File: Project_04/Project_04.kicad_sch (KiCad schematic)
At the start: 1 part, among them U1 74AUC2G79

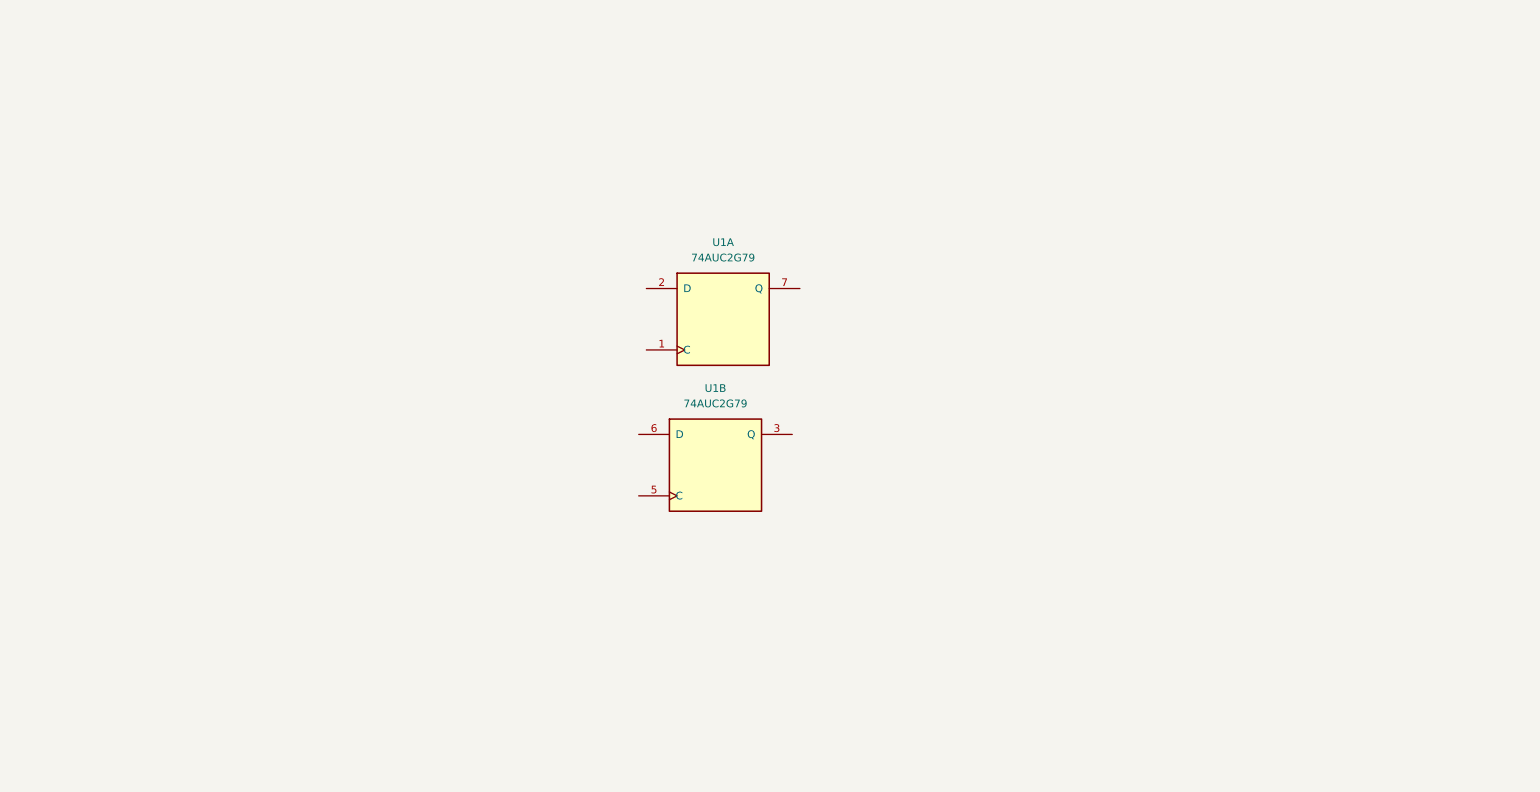
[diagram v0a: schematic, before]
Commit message: some changes
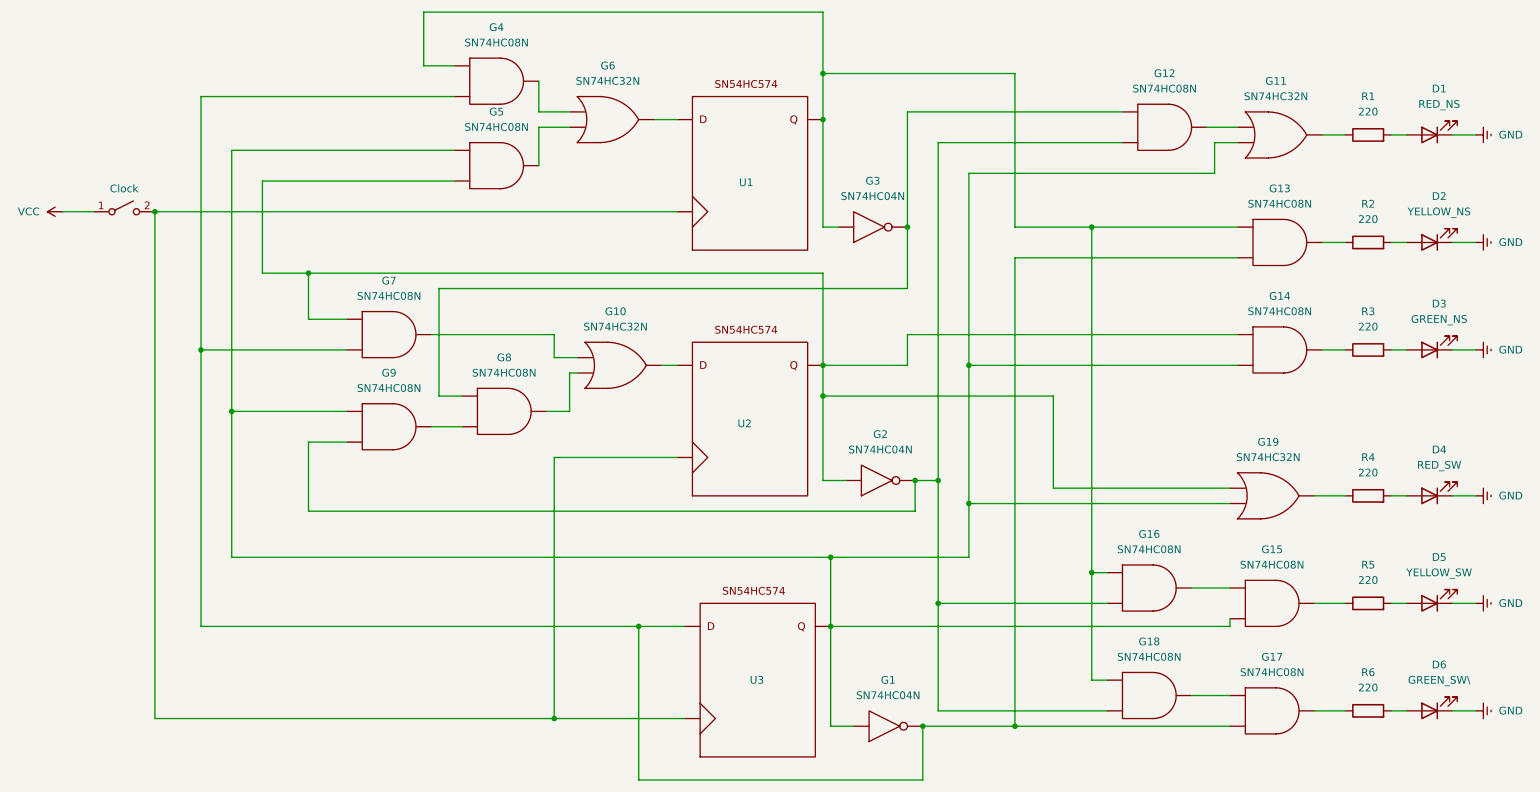
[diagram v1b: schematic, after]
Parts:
- removed U1: 74AUC2G79, symbol 74xGxx:74AUC2G79
- added D1: RED_NS, symbol Device:LED
- added D2: YELLOW_NS, symbol Device:LED
- added D3: GREEN_NS, symbol Device:LED
- added D4: RED_SW, symbol Device:LED
- added D5: YELLOW_SW, symbol Device:LED
- added D6: GREEN_SW\, symbol Device:LED
- added G1, G2, G3: SN74HC04N, symbol MDSD symbols:Inverter
- added G10, G11, G19, G6: SN74HC32N, symbol MDSD symbols:OR_gate
- added G12, G13, G14, G15, G16, G17, G18, G4, G5, G7, G8, G9: SN74HC08N, symbol MDSD symbols:AND_gate
- added R1, R2, R3, R4, R5, R6: 220, symbol Device:R
- added SW1: Clock, symbol Switch:SW_SPST
- added U1, U2, U3: ~, symbol MDSD symbols:d_flip_flop_2
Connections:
- new net: SW1.2 (B), U1., U2., U3.
- new net: G4., G6.
- new net: G6., U1.
- new net: G5., G6.
- new net: G1., G11., G14., G15., G19., G5., G9., U3.
- new net: G1., G13., G17., G4., G7., U3.
- new net: G19., R4.1
- new net: D4.2 (A), R4.2
- new net: G17., R6.1
- new net: D6.2 (A), R6.2
- new net: G12., G16., G18., G2., G9.
- new net: G13., G16., G18., G3., G4., U1.
- new net: G15., G16.
- new net: D1.2 (A), R1.2
- new net: G12., G3., G8.
- new net: G11., G12.
- new net: G14., R3.1
- new net: D3.2 (A), R3.2
- new net: G15., R5.1
- new net: D5.2 (A), R5.2
- new net: G14., G19., G2., G5., G7., U2.
- new net: G10., G7.
- new net: G11., R1.1
- new net: G17., G18.
- new net: G8., G9.
- new net: G13., R2.1
- new net: G10., G8.
- new net: G10., U2.
- new net: D2.2 (A), R2.2
- new net GND: D1.1 (K), D2.1 (K), D3.1 (K), D4.1 (K), D5.1 (K), D6.1 (K)
- new net VCC: SW1.1 (A)
